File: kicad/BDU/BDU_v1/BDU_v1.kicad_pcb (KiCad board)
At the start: 2 copper layers, 2 parts, among them U1 LTV-847S, U2 TRA3-1212

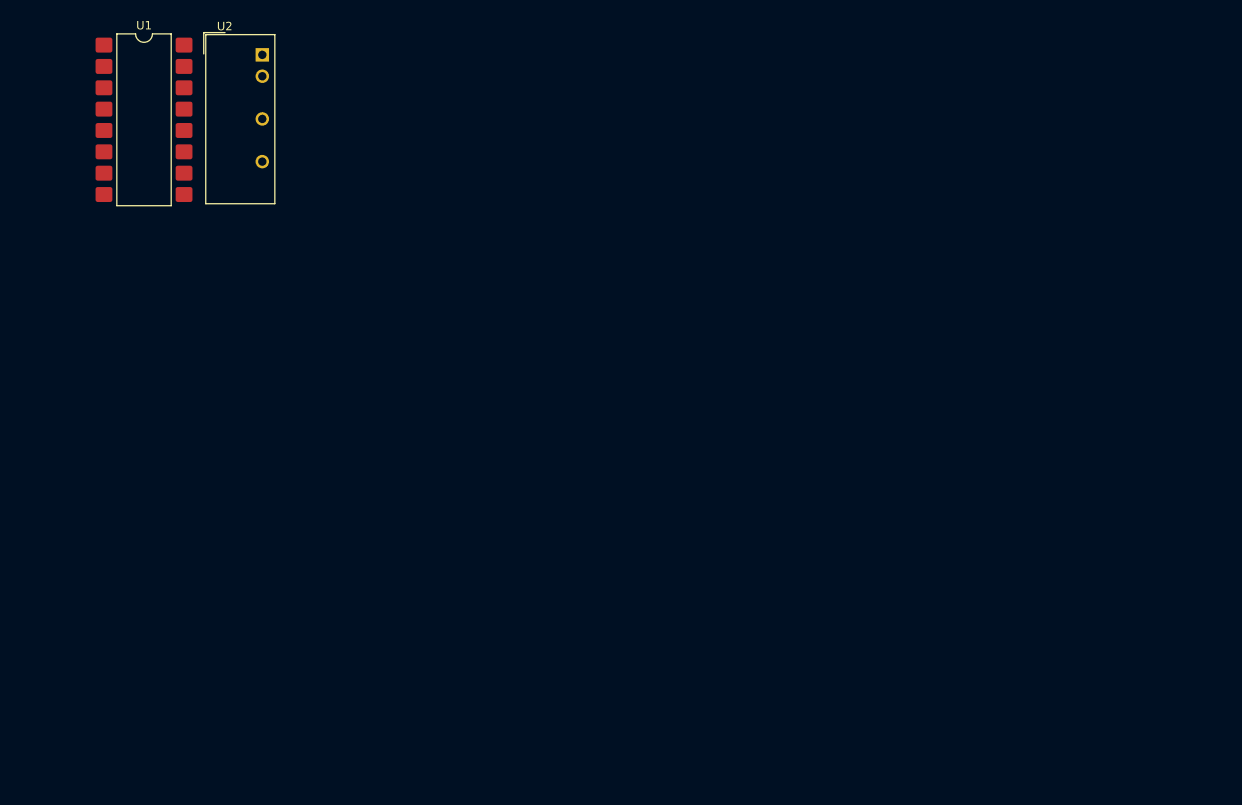
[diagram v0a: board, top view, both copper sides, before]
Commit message: BDU
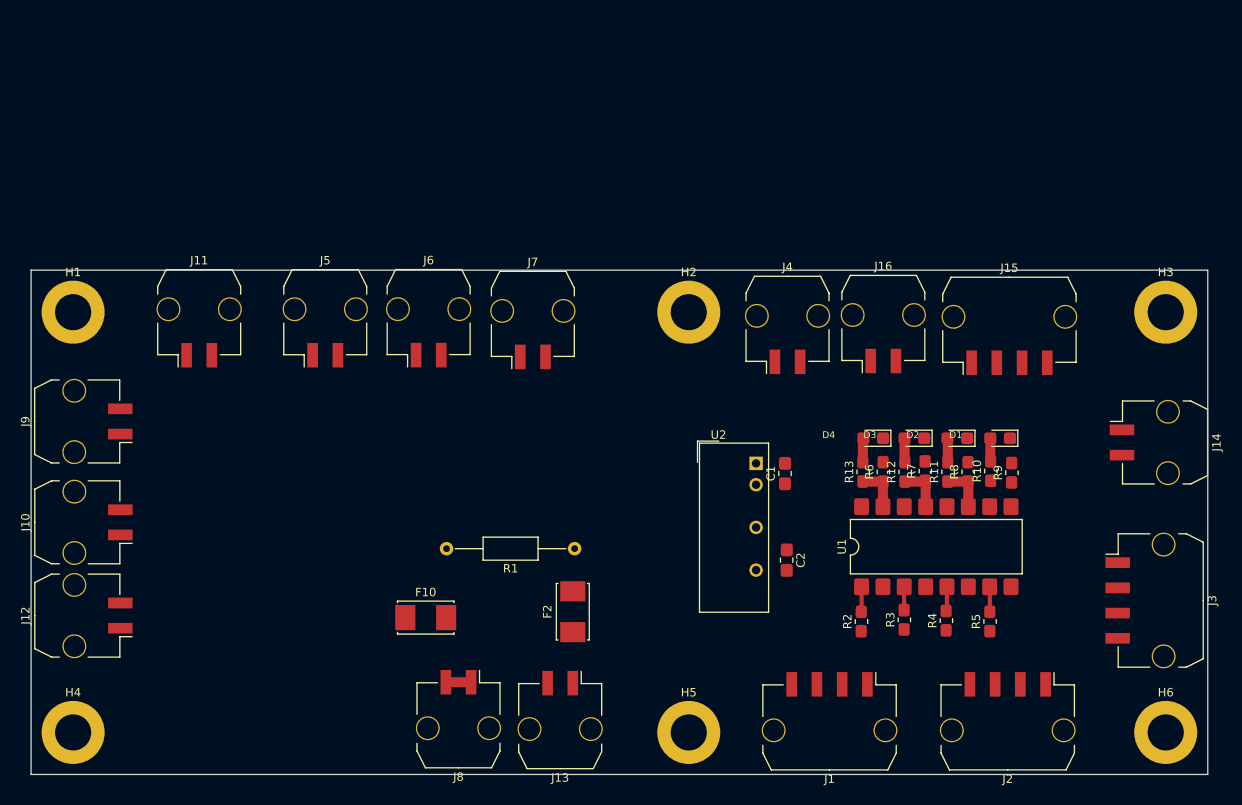
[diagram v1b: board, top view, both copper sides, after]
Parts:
- added C1: 2.2uF, RMC_Capacitor:C_0805_2012Metric_Pad1.18x1.45mm_HandSolder_L, F.Cu at (169.7, 94.2)
- added C2: 1uF, RMC_Capacitor:C_0805_2012Metric_Pad1.18x1.45mm_HandSolder_L, F.Cu at (169.9, 104.5)
- added D1: LED, RMC_LED:LED_0805_2012Metric_Pad1.45x1.40mm_HandSolder, F.Cu at (195.3, 90.0)
- added D2: LED, RMC_LED:LED_0805_2012Metric_Pad1.45x1.40mm_HandSolder, F.Cu at (190.2, 90.0)
- added D3: LED, RMC_LED:LED_0805_2012Metric_Pad1.45x1.40mm_HandSolder, F.Cu at (185.1, 90.0)
- added D4: LED, RMC_LED:LED_0805_2012Metric_Pad1.45x1.40mm_HandSolder, F.Cu at (180.2, 90.0)
- added F10: Fuse, Fuse:Fuseholder_Littelfuse_Nano2_157x, F.Cu at (127.0, 111.3)
- added F2: Fuse, Fuse:Fuseholder_Littelfuse_Nano2_157x, F.Cu at (144.4, 110.6)
- added H1: MountingHole_Pad, MountingHole:MountingHole_4.3mm_M4_DIN965_Pad, F.Cu at (85.0, 75.0)
- added H2: MountingHole_Pad, MountingHole:MountingHole_4.3mm_M4_DIN965_Pad, F.Cu at (158.2, 75.0)
- added H3: MountingHole_Pad, MountingHole:MountingHole_4.3mm_M4_DIN965_Pad, F.Cu at (215.0, 75.0)
- added H4: MountingHole_Pad, MountingHole:MountingHole_4.3mm_M4_DIN965_Pad, F.Cu at (85.0, 125.0)
- added H5: MountingHole_Pad, MountingHole:MountingHole_4.3mm_M4_DIN965_Pad, F.Cu at (158.2, 125.0)
- added H6: MountingHole_Pad, MountingHole:MountingHole_4.3mm_M4_DIN965_Pad, F.Cu at (215.0, 125.0)
- added J1: Relay connector, Connector_Molex:Molex_Micro-Fit_3.0_43650-0410_1x04-1MP_P3.00mm_Horizontal_PnP, F.Cu at (175.0, 124.4)
- added J10: Voltmeter-, Connector_Molex:Molex_Micro-Fit_3.0_43650-0210_1x02-1MP_P3.00mm_Horizontal_PnP, F.Cu at (85.5, 100.0)
- added J11: IMD-, Connector_Molex:Molex_Micro-Fit_3.0_43650-0210_1x02-1MP_P3.00mm_Horizontal_PnP, F.Cu at (100.0, 75.0)
- added J12: AIR-, Connector_Molex:Molex_Micro-Fit_3.0_43650-0210_1x02-1MP_P3.00mm_Horizontal_PnP, F.Cu at (85.5, 111.1)
- added J13: AIR+, Connector_Molex:Molex_Micro-Fit_3.0_43650-0210_1x02-1MP_P3.00mm_Horizontal_PnP, F.Cu at (142.9, 124.2)
- added J14: AIR+, Connector_Molex:Molex_Micro-Fit_3.0_43650-0210_1x02-1MP_P3.00mm_Horizontal_PnP, F.Cu at (214.9, 90.5)
- added J15: AMS, Connector_Molex:Molex_Micro-Fit_3.0_43650-0410_1x04-1MP_P3.00mm_Horizontal_PnP, F.Cu at (196.4, 75.9)
- added J16: DCDC, Connector_Molex:Molex_Micro-Fit_3.0_43650-0210_1x02-1MP_P3.00mm_Horizontal_PnP, F.Cu at (181.4, 75.7)
- added J2: Relay connector, Connector_Molex:Molex_Micro-Fit_3.0_43650-0410_1x04-1MP_P3.00mm_Horizontal_PnP, F.Cu at (196.2, 124.4)
- added J3: Relay connector, Connector_Molex:Molex_Micro-Fit_3.0_43650-0410_1x04-1MP_P3.00mm_Horizontal_PnP, F.Cu at (214.4, 109.3)
- added J4: Conn_01x02, Connector_Molex:Molex_Micro-Fit_3.0_43650-0210_1x02-1MP_P3.00mm_Horizontal_PnP, F.Cu at (170.0, 75.8)
- added J5: IMD+, Connector_Molex:Molex_Micro-Fit_3.0_43650-0210_1x02-1MP_P3.00mm_Horizontal_PnP, F.Cu at (115.0, 75.0)
- added J6: Voltmeter+, Connector_Molex:Molex_Micro-Fit_3.0_43650-0210_1x02-1MP_P3.00mm_Horizontal_PnP, F.Cu at (127.3, 75.0)
- added J7: TSAL_green+, Connector_Molex:Molex_Micro-Fit_3.0_43650-0210_1x02-1MP_P3.00mm_Horizontal_PnP, F.Cu at (139.7, 75.2)
- added J8: AIR+, Connector_Molex:Molex_Micro-Fit_3.0_43650-0210_1x02-1MP_P3.00mm_Horizontal_PnP, F.Cu at (130.8, 124.2)
- added J9: TSAL_green-, Connector_Molex:Molex_Micro-Fit_3.0_43650-0210_1x02-1MP_P3.00mm_Horizontal_PnP, F.Cu at (85.5, 88.0)
- added R1: 3K9, Resistor_THT:R_Axial_DIN0207_L6.3mm_D2.5mm_P15.24mm_Horizontal, F.Cu at (144.7, 103.1)
- added R10: 1k, RMC_Resistor:R_0805_2012Metric_Pad1.20x1.40mm_HandSolder_L, F.Cu at (194.2, 93.9)
- added R11: 1k, RMC_Resistor:R_0805_2012Metric_Pad1.20x1.40mm_HandSolder_L, F.Cu at (189.1, 94.0)
- added R12: 1k, RMC_Resistor:R_0805_2012Metric_Pad1.20x1.40mm_HandSolder_L, F.Cu at (184.0, 94.0)
- added R13: 1k, RMC_Resistor:R_0805_2012Metric_Pad1.20x1.40mm_HandSolder_L, F.Cu at (179.0, 94.0)
- added R2: 1k, RMC_Resistor:R_0805_2012Metric_Pad1.20x1.40mm_HandSolder_L, F.Cu at (178.8, 111.8)
- added R3: 1k, RMC_Resistor:R_0805_2012Metric_Pad1.20x1.40mm_HandSolder_L, F.Cu at (183.9, 111.6)
- added R4: 1k, RMC_Resistor:R_0805_2012Metric_Pad1.20x1.40mm_HandSolder_L, F.Cu at (188.9, 111.7)
- added R5: 1k, RMC_Resistor:R_0805_2012Metric_Pad1.20x1.40mm_HandSolder_L, F.Cu at (194.1, 111.8)
- added R6: 4k7, RMC_Resistor:R_0805_2012Metric_Pad1.20x1.40mm_HandSolder_L, F.Cu at (181.4, 94.0)
- added R7: 4k7, RMC_Resistor:R_0805_2012Metric_Pad1.20x1.40mm_HandSolder_L, F.Cu at (186.4, 93.9)
- added R8: 4k7, RMC_Resistor:R_0805_2012Metric_Pad1.20x1.40mm_HandSolder_L, F.Cu at (191.5, 94.0)
- added R9: 4k7, RMC_Resistor:R_0805_2012Metric_Pad1.20x1.40mm_HandSolder_L, F.Cu at (196.7, 94.1)
- moved U1 107.1 mm to (187.7, 102.9), turned to 90 degrees
- moved U2 76.2 mm to (166.3, 93.0)
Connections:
- U1 pad 11: unconnected-(U1-Pad11) -> /pre_out
- U1 pad 13: unconnected-(U1-Pad13) -> /low_out
- U1 pad 15: unconnected-(U1-Pad15) -> /high_out
- U1 pad 8: GND -> PRE-
- U1 pad 9: unconnected-(U1-Pad9) -> /sdc_out
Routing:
- net /low_out: track 0.00 -> 5.55 mm
- net /pre_out: track 0.00 -> 5.40 mm
- net /high_out: track 0.00 -> 5.39 mm
- net Net-(R2-Pad2): track 0.00 -> 3.00 mm
- net TS+: track 0.00 -> 3.00 mm
- net Net-(R5-Pad2): track 0.00 -> 2.99 mm
- net Net-(R4-Pad2): track 0.00 -> 2.92 mm
- net Net-(D4-A): track 0.00 -> 2.87 mm
- net Net-(D3-A): track 0.00 -> 2.87 mm
- net Net-(D2-A): track 0.00 -> 2.87 mm
- net Net-(R3-Pad2): track 0.00 -> 2.79 mm
- net Net-(D1-A): track 0.00 -> 2.77 mm
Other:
- board outline added: 140 x 60 mm
